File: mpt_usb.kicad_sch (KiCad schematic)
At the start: 8 parts, among them J101 USB4105GFA120, U101 RCLAMP0854P.TCT

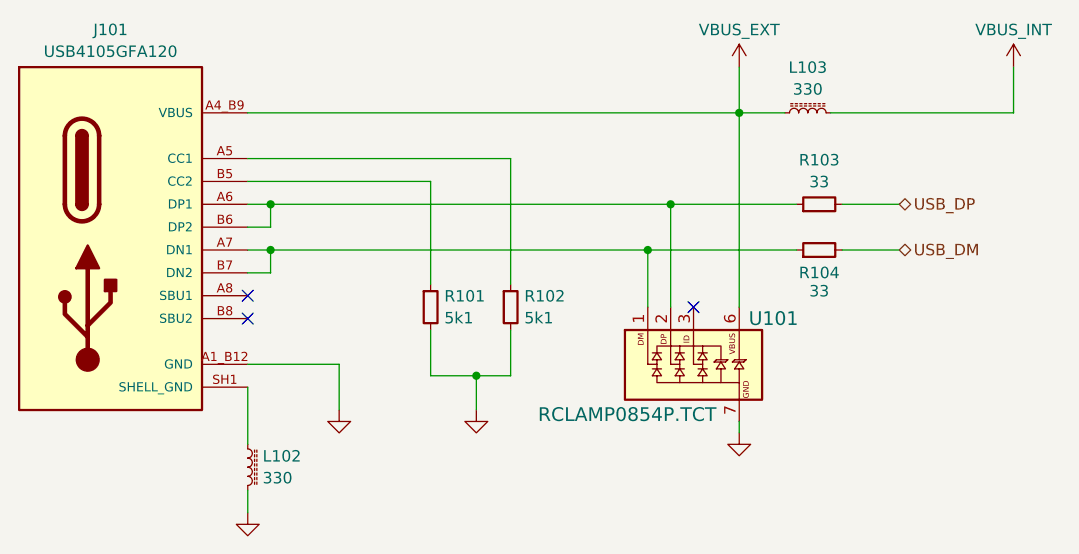
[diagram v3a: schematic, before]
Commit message: Added Display
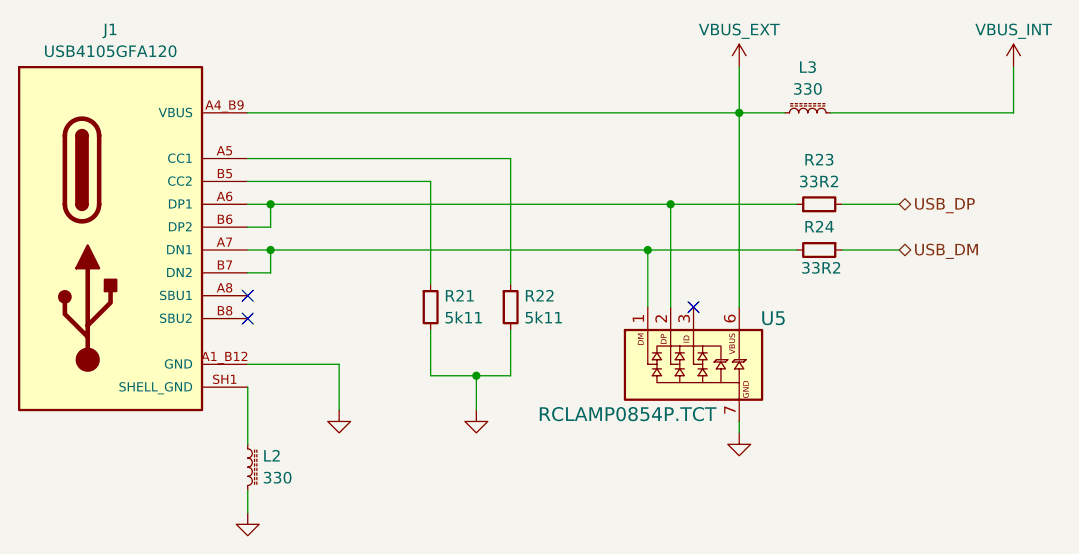
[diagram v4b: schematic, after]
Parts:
- R21: renamed from R101; value 5k1 -> 5k11; symbol db:resistor/00.018.0009.0018 -> db:resistor_0603/00.018.0009.0520; Dist1# 311-5.10KHRCT-ND -> 311-5.11KHRCT-ND; MFR# RC0603FR-075K1L -> RC0603FR-075K11L; Modified 2026-03-22 16:51:27 -> 2026-10-07 14:47:41; Rating 100mW, 1% -> 125mW, 1%; Remarks (none) -> Autogenerated; Version 1 -> 2
- R22: renamed from R102; value 5k1 -> 5k11; symbol db:resistor/00.018.0009.0018 -> db:resistor_0603/00.018.0009.0520; Dist1# 311-5.10KHRCT-ND -> 311-5.11KHRCT-ND; MFR# RC0603FR-075K1L -> RC0603FR-075K11L; Modified 2026-03-22 16:51:27 -> 2026-10-07 14:47:41; Rating 100mW, 1% -> 125mW, 1%; Remarks (none) -> Autogenerated; Version 1 -> 2
- R23: renamed from R103; value 33 -> 33R2; symbol db:resistor/00.018.0009.0019 -> db:resistor_0603/00.018.0009.0393; Dist1# 13-RC0603FR-0733RLCT-ND -> 311-33.2HRCT-ND; MFR# RC0603FR-0733RL -> RC0603FR-0733R2L; Modified 2026-03-22 16:53:08 -> 2026-10-07 14:47:41; Rating 100mW, 1% -> 125mW, 1%; Remarks (none) -> Autogenerated; Version 1 -> 2
- R24: renamed from R104; value 33 -> 33R2; symbol db:resistor/00.018.0009.0019 -> db:resistor_0603/00.018.0009.0393; Dist1# 13-RC0603FR-0733RLCT-ND -> 311-33.2HRCT-ND; MFR# RC0603FR-0733RL -> RC0603FR-0733R2L; Modified 2026-03-22 16:53:08 -> 2026-10-07 14:47:41; Rating 100mW, 1% -> 125mW, 1%; Remarks (none) -> Autogenerated; Version 1 -> 2
- renumbered J101 to J1, L102 to L2, L103 to L3, U101 to U5
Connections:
- net USB_DM: now also R24.1; no longer R24.2
- net at J1.A7 (DN1), J1.B7 (DN2), U5.1 (DM): now also R24.2; no longer R24.1
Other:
- moved on the sheet: R24
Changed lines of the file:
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@@
 		(dnp no)
 		(fields_autoplaced yes)
-		(property "Reference" "L103"
+		(property "Reference" "L3"
 			(at 167.64 66.0865 90)
 			(show_name no)
@@
 			(project "MPT"
 				(path "/328ebaa0-d01b-4b80-b614-bb0154e8d306/fccb15cc-77d6-497f-b3d6-022c5206b90a"
-					(reference "L103")
+					(reference "L3")
 					(unit 1)
 				)
@@
 		(dnp no)
 		(fields_autoplaced yes)
-		(property "Reference" "#PWR0111"
+		(property "Reference" "#PWR038"
 			(at 115.57 110.49 0)
 			(hide yes)
@@
 			(project "MPT"
 				(path "/328ebaa0-d01b-4b80-b614-bb0154e8d306/fccb15cc-77d6-497f-b3d6-022c5206b90a"
-					(reference "#PWR0111")
+					(reference "#PWR038")
 					(unit 1)
 				)
@@
 		(dnp no)
 		(fields_autoplaced yes)
-		(property "Reference" "#PWR0117"
+		(property "Reference" "#PWR042"
 			(at 190.5 69.85 0)
 			(hide yes)
@@
 			(project "MPT"
 				(path "/328ebaa0-d01b-4b80-b614-bb0154e8d306/fccb15cc-77d6-497f-b3d6-022c5206b90a"
-					(reference "#PWR0117")
+					(reference "#PWR042")
 					(unit 1)
 				)
@@
 		(dnp no)
 		(fields_autoplaced yes)
-		(property "Reference" "#PWR0112"
+		(property "Reference" "#PWR037"
 			(at 105.41 121.92 0)
 			(hide yes)
@@
 			(project "MPT"
 				(path "/328ebaa0-d01b-4b80-b614-bb0154e8d306/fccb15cc-77d6-497f-b3d6-022c5206b90a"
-					(reference "#PWR0112")
+					(reference "#PWR037")
 					(unit 1)
 				)
@@
 	)
 	(symbol
-		(lib_id "db:resistor/00.018.0009.0018")
+		(lib_id "db:resistor_0603/00.018.0009.0520")
 		(at 125.73 92.71 0)
 		(unit 1)
@@
 		(dnp no)
 		(fields_autoplaced yes)
-		(property "Reference" "R101"
+		(property "Reference" "R21"
 			(at 127.254 91.4978 0)
 			(show_name no)
@@
 			)
 		)
-		(property "Value" "5k1"
+		(property "Value" "5k11"
 			(at 127.254 93.9221 0)
 			(show_name no)
@@
 			)
 		)
-		(property "Description" ""
+		(property "Description" "R 5k11 0603"
 			(at 125.73 92.71 0)
 			(hide yes)
@@
 			)
 		)
-		(property "MFR#" "RC0603FR-075K1L"
+		(property "MFR#" "RC0603FR-075K11L"
 			(at 125.73 92.71 0)
 			(hide yes)
@@
 			)
 		)
-		(property "Rating" "100mW, 1%"
+		(property "Rating" "125mW, 1%"
 			(at 125.73 92.71 0)
 			(hide yes)
@@
 			)
 		)
-		(property "Remarks" ""
+		(property "Remarks" "Autogenerated"
 			(at 125.73 92.71 0)
 			(hide yes)
@@
 			)
 		)
-		(property "Dist1#" "311-5.10KHRCT-ND"
+		(property "Dist1#" "311-5.11KHRCT-ND"
 			(at 125.73 92.71 0)
 			(hide yes)
@@
 			)
 		)
-		(property "Version" "1"
+		(property "Version" "2"
 			(at 125.73 92.71 0)
 			(hide yes)
@@
 			)
 		)
-		(property "Modified" "2026-03-22 16:51:27"
+		(property "Modified" "2026-10-07 14:47:41"
 			(at 125.73 92.71 0)
 			(hide yes)
@@
 			(project "MPT"
 				(path "/328ebaa0-d01b-4b80-b614-bb0154e8d306/fccb15cc-77d6-497f-b3d6-022c5206b90a"
-					(reference "R101")
+					(reference "R21")
 					(unit 1)
 				)
@@
 		(dnp no)
 		(fields_autoplaced yes)
-		(property "Reference" "J101"
+		(property "Reference" "J1"
 			(at 90.17 61.8955 0)
 			(show_name no)
@@
 			(project "MPT"
 				(path "/328ebaa0-d01b-4b80-b614-bb0154e8d306/fccb15cc-77d6-497f-b3d6-022c5206b90a"
-					(reference "J101")
+					(reference "J1")
 					(unit 1)
 				)
@@
 		(dnp no)
 		(fields_autoplaced yes)
-		(property "Reference" "#PWR0110"
+		(property "Reference" "#PWR039"
 			(at 130.81 110.49 0)
 			(hide yes)
@@
 			(project "MPT"
 				(path "/328ebaa0-d01b-4b80-b614-bb0154e8d306/fccb15cc-77d6-497f-b3d6-022c5206b90a"
-					(reference "#PWR0110")
+					(reference "#PWR039")
 					(unit 1)
 				)
@@
 		(dnp no)
 		(fields_autoplaced yes)
-		(property "Reference" "L102"
+		(property "Reference" "L2"
 			(at 107.061 109.2778 0)
 			(show_name no)
@@
 			(project "MPT"
 				(path "/328ebaa0-d01b-4b80-b614-bb0154e8d306/fccb15cc-77d6-497f-b3d6-022c5206b90a"
-					(reference "L102")
+					(reference "L2")
 					(unit 1)
 				)
@@
 		(dnp no)
 		(fields_autoplaced yes)
-		(property "Reference" "#PWR0113"
+		(property "Reference" "#PWR041"
 			(at 160.02 113.03 0)
 			(hide yes)
@@
 			(project "MPT"
 				(path "/328ebaa0-d01b-4b80-b614-bb0154e8d306/fccb15cc-77d6-497f-b3d6-022c5206b90a"
-					(reference "#PWR0113")
+					(reference "#PWR041")
 					(unit 1)
 				)
@@
 	)
 	(symbol
-		(lib_id "db:resistor/00.018.0009.0018")
+		(lib_id "db:resistor_0603/00.018.0009.0520")
 		(at 134.62 92.71 0)
 		(unit 1)
@@
 		(dnp no)
 		(fields_autoplaced yes)
-		(property "Reference" "R102"
+		(property "Reference" "R22"
 			(at 136.144 91.4978 0)
 			(show_name no)
@@
 			)
 		)
-		(property "Value" "5k1"
+		(property "Value" "5k11"
 			(at 136.144 93.9221 0)
 			(show_name no)
@@
 			)
 		)
-		(property "Description" ""
+		(property "Description" "R 5k11 0603"
 			(at 134.62 92.71 0)
 			(hide yes)
@@
 			)
 		)
-		(property "MFR#" "RC0603FR-075K1L"
+		(property "MFR#" "RC0603FR-075K11L"
 			(at 134.62 92.71 0)
 			(hide yes)
@@
 			)
 		)
-		(property "Rating" "100mW, 1%"
+		(property "Rating" "125mW, 1%"
 			(at 134.62 92.71 0)
 			(hide yes)
@@
 			)
 		)
-		(property "Remarks" ""
+		(property "Remarks" "Autogenerated"
 			(at 134.62 92.71 0)
 			(hide yes)
@@
 			)
 		)
-		(property "Dist1#" "311-5.10KHRCT-ND"
+		(property "Dist1#" "311-5.11KHRCT-ND"
 			(at 134.62 92.71 0)
 			(hide yes)
@@
 			)
 		)
-		(property "Version" "1"
+		(property "Version" "2"
 			(at 134.62 92.71 0)
 			(hide yes)
@@
 			)
 		)
-		(property "Modified" "2026-03-22 16:51:27"
+		(property "Modified" "2026-10-07 14:47:41"
 			(at 134.62 92.71 0)
 			(hide yes)
@@
 			(project "MPT"
 				(path "/328ebaa0-d01b-4b80-b614-bb0154e8d306/fccb15cc-77d6-497f-b3d6-022c5206b90a"
-					(reference "R102")
+					(reference "R22")
 					(unit 1)
 				)
@@
 		(dnp no)
 		(fields_autoplaced yes)
-		(property "Reference" "#PWR0116"
+		(property "Reference" "#PWR040"
 			(at 160.02 69.85 0)
 			(hide yes)
@@
 			(project "MPT"
 				(path "/328ebaa0-d01b-4b80-b614-bb0154e8d306/fccb15cc-77d6-497f-b3d6-022c5206b90a"
-					(reference "#PWR0116")
+					(reference "#PWR040")
 					(unit 1)
 				)
@@
 	)
 	(symbol
-		(lib_id "db:resistor/00.018.0009.0019")
+		(lib_id "db:resistor_0603/00.018.0009.0393")
 		(at 168.91 81.28 90)
 		(unit 1)
@@
 		(dnp no)
 		(fields_autoplaced yes)
-		(property "Reference" "R103"
+		(property "Reference" "R23"
 			(at 168.91 76.3735 90)
 			(show_name no)
@@
 			)
 		)
-		(property "Value" "33"
+		(property "Value" "33R2"
 			(at 168.91 78.7978 90)
 			(show_name no)
@@
 			)
 		)
-		(property "Description" ""
+		(property "Description" "R 33R2 0603"
 			(at 168.91 81.28 0)
 			(hide yes)
@@
 			)
 		)
-		(property "MFR#" "RC0603FR-0733RL"
+		(property "MFR#" "RC0603FR-0733R2L"
 			(at 168.91 81.28 0)
 			(hide yes)
@@
 			)
 		)
-		(property "Rating" "100mW, 1%"
+		(property "Rating" "125mW, 1%"
 			(at 168.91 81.28 0)
 			(hide yes)
@@
 			)
 		)
-		(property "Remarks" ""
+		(property "Remarks" "Autogenerated"
 			(at 168.91 81.28 0)
 			(hide yes)
@@
 			)
 		)
-		(property "Dist1#" "13-RC0603FR-0733RLCT-ND"
+		(property "Dist1#" "311-33.2HRCT-ND"
 			(at 168.91 81.28 0)
 			(hide yes)
@@
 			)
 		)
-		(property "Version" "1"
+		(property "Version" "2"
 			(at 168.91 81.28 0)
 			(hide yes)
@@
 			)
 		)
-		(property "Modified" "2026-03-22 16:53:08"
+		(property "Modified" "2026-10-07 14:47:41"
 			(at 168.91 81.28 0)
 			(hide yes)
@@
 			(project "MPT"
 				(path "/328ebaa0-d01b-4b80-b614-bb0154e8d306/fccb15cc-77d6-497f-b3d6-022c5206b90a"
-					(reference "R103")
+					(reference "R23")
 					(unit 1)
 				)
@@
 	)
 	(symbol
-		(lib_id "db:resistor/00.018.0009.0019")
-		(at 168.91 86.36 90)
+		(lib_id "db:resistor_0603/00.018.0009.0393")
+		(at 168.91 86.36 270)
 		(unit 1)
 		(body_style 1)
@@
 		(in_pos_files yes)
 		(dnp no)
-		(property "Reference" "R104"
-			(at 168.91 88.9 90)
-			(show_name no)
-			(do_not_autoplace no)
-			(effects
-				(font
-					(size 1.27 1.27)
-				)
-			)
-		)
-		(property "Value" "33"
-			(at 168.91 90.932 90)
-			(show_name no)
-			(do_not_autoplace no)
-			(effects
-				(font
-					(size 1.27 1.27)
-				)
+		(property "Reference" "R24"
+			(at 168.91 83.82 90)
+			(show_name no)
+			(do_not_autoplace no)
+			(effects
+				(font
+					(size 1.27 1.27)
+				)
+			)
+		)
+		(property "Value" "33R2"
+			(at 166.878 88.392 90)
+			(show_name no)
+			(do_not_autoplace no)
+			(effects
+				(font
+					(size 1.27 1.27)
+				)
+				(justify left)
 			)
 		)
@@
 			)
 		)
-		(property "Description" ""
+		(property "Description" "R 33R2 0603"
 			(at 168.91 86.36 0)
 			(hide yes)
@@
 			)
 		)
-		(property "MFR#" "RC0603FR-0733RL"
+		(property "MFR#" "RC0603FR-0733R2L"
 			(at 168.91 86.36 0)
 			(hide yes)
@@
 			)
 		)
-		(property "Rating" "100mW, 1%"
+		(property "Rating" "125mW, 1%"
 			(at 168.91 86.36 0)
 			(hide yes)
@@
 			)
 		)
-		(property "Remarks" ""
+		(property "Remarks" "Autogenerated"
 			(at 168.91 86.36 0)
 			(hide yes)
@@
 			)
 		)
-		(property "Dist1#" "13-RC0603FR-0733RLCT-ND"
+		(property "Dist1#" "311-33.2HRCT-ND"
 			(at 168.91 86.36 0)
 			(hide yes)
@@
 			)
 		)
-		(property "Version" "1"
+		(property "Version" "2"
 			(at 168.91 86.36 0)
 			(hide yes)
@@
 			)
 		)
-		(property "Modified" "2026-03-22 16:53:08"
+		(property "Modified" "2026-10-07 14:47:41"
 			(at 168.91 86.36 0)
 			(hide yes)
@@
 			(project "MPT"
 				(path "/328ebaa0-d01b-4b80-b614-bb0154e8d306/fccb15cc-77d6-497f-b3d6-022c5206b90a"
-					(reference "R104")
+					(reference "R24")
 					(unit 1)
 				)
@@
 		(in_pos_files yes)
 		(dnp no)
-		(property "Reference" "U101"
+		(property "Reference" "U5"
 			(at 163.83 93.98 0)
 			(show_name no)
@@
 			(project "MPT"
 				(path "/328ebaa0-d01b-4b80-b614-bb0154e8d306/fccb15cc-77d6-497f-b3d6-022c5206b90a"
-					(reference "U101")
+					(reference "U5")
 					(unit 1)
 				)
